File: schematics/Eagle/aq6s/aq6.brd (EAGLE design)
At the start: 99.8 x 66.8 mm, 24 parts

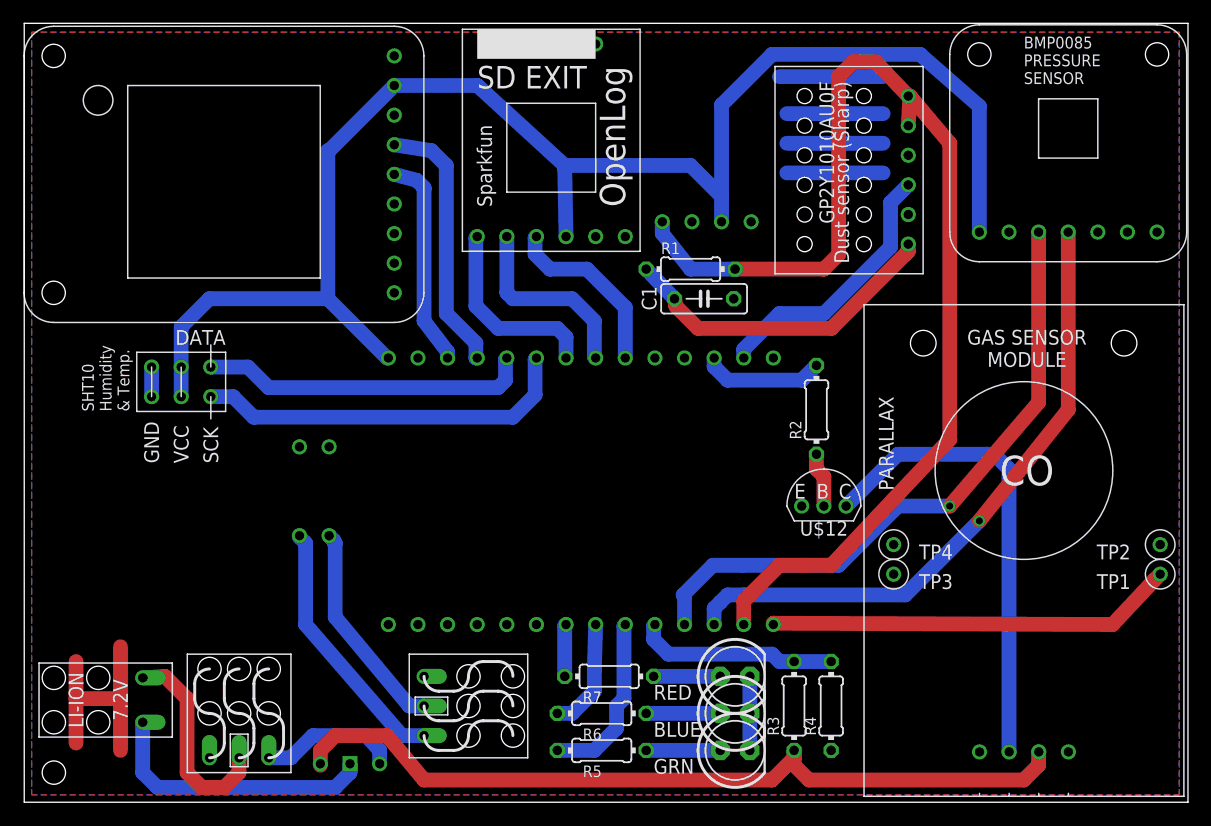
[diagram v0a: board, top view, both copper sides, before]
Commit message: pcb images
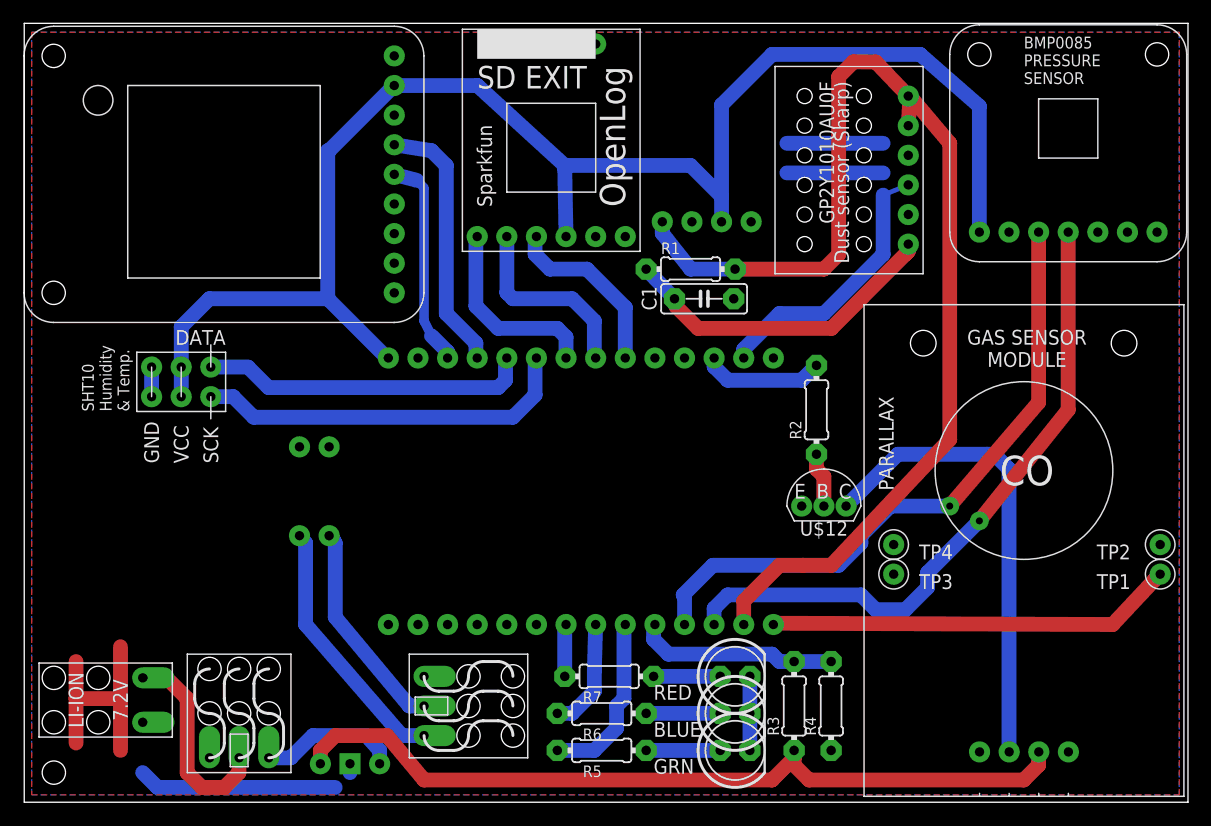
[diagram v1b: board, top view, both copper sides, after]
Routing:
- net GND: track 86.1 -> 62.9 mm
- net N$24: track 54.7 -> 56.5 mm
- net N$1: track 22.9 -> 23.5 mm
